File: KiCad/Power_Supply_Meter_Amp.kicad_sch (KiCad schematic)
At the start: 630 parts, among them J1 R_Phono_In, J10 VCC_IN, J11 VCC_OUT, J12 EMK_In, J13 EMK_Out, J14 EMK_Out, J15 Mic_Effekt_Out, J16 Mic_Effekt_Out, J17 Mic_Effekt_Out, J18 Mic_Effekt_Out, J19 Phono/Line_Out, J2 L_Phono_In, J20 Mic_Effekt_Out, J21 Conn_01x05_bridged, J22 EMK_In, J24 Mic_Effekt_In, J25 Mic_Effekt_In, J26 Phono/Line_In, J27 Mic_Effekt_In, J28 Pegel_Out, J29 Pegel_Out, J3 R_Line_In, J30 Pegel_In, J31 Pegel_In, J32 Pegel_In, J33 Pegel_In, J34 LED_Out, J35 LED_In, J36 VU_Meter_Out, J37 AUX_Send_3, J38 AUX_Send_1, J39 AUX_Send_2, J4 L_Line_In, J40 Bass_Out, J41 Kick_Out, J42 Mid_Out, J43 High_Out, J44 Line_Out_L, J45 Line_Out_R, J5 Mic_In, J6 Effekt_In, J7 AUX_RET_1, J8 AUX_RET_2, J9 AUX_RET_3, SW1 SW_DPST, SW10 SW_SPDT, SW11 SW_SPDT, SW12 SW_SPDT, SW2 SW_SPDT, SW3 SW_SPDT, SW4 SW_SPDT, SW5 SW_SPDT, SW6 SW_SPDT, SW7 SW_SPDT, SW8 SW_SPDT, SW9 SW_Rotary_1x4, U1 TL074, U10 TL074, U11 TL074, U12 TL074, U13 TL074, U14 TL074, U15 TL074, U16 TL074, U17 TL074, U18 TL074, U19 TL074, U2 TL074, U20 TL074, U21 TL074, U22 TL074, U23 TL074, U24 TL074, U25 INA128U, U3 TL074, U4 TL074, U5 TL074, U6 REC10K-2409, U7 REC10K-2415, U8 TL074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

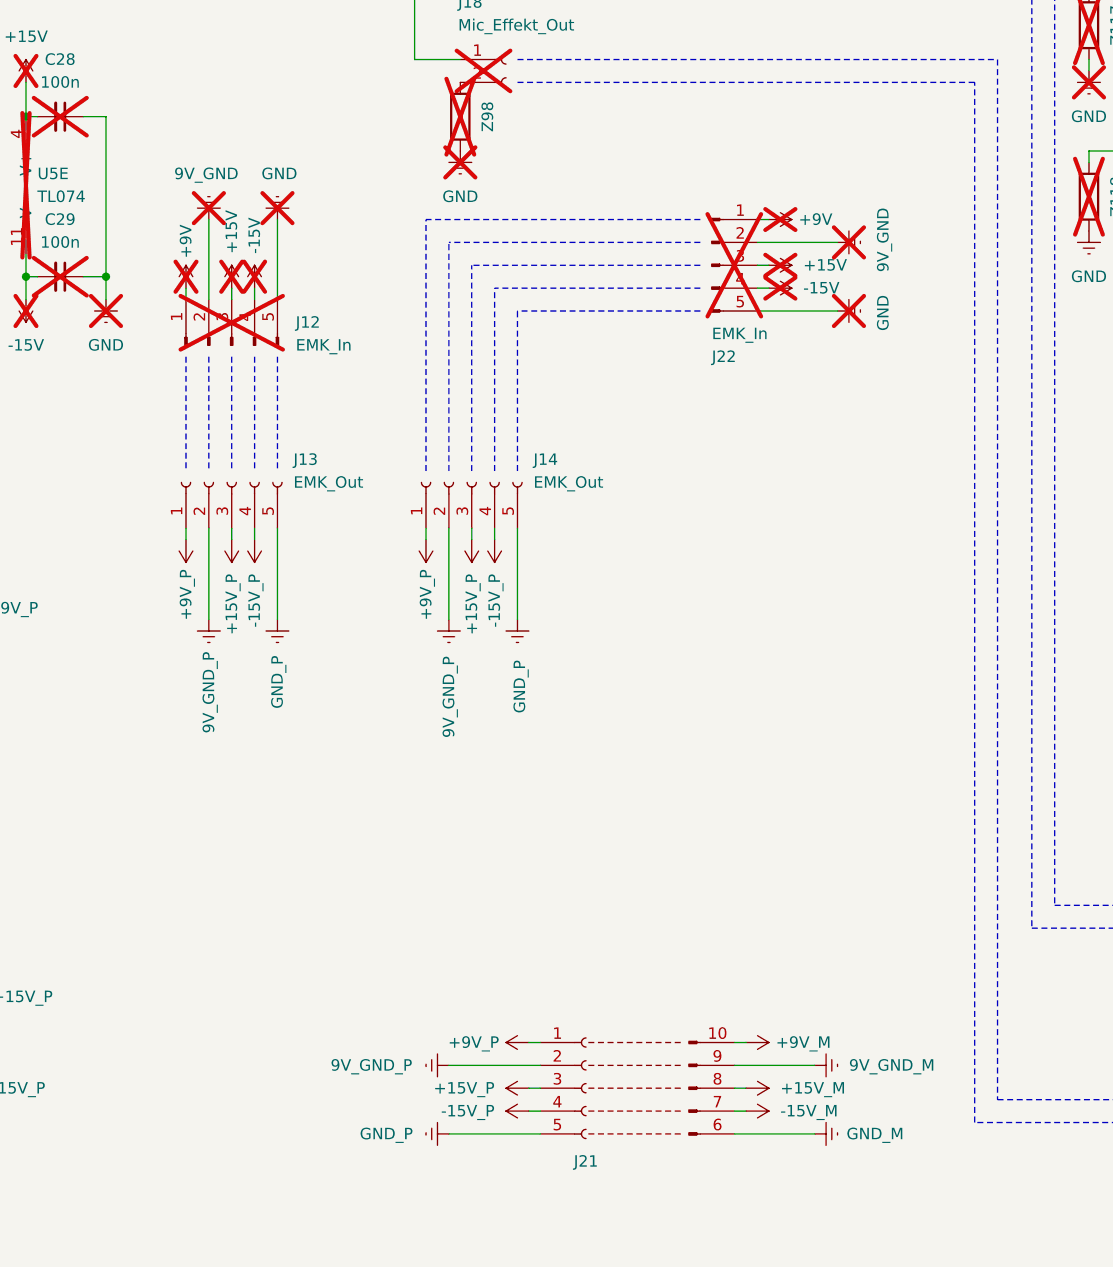
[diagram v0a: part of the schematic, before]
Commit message: PCB Update
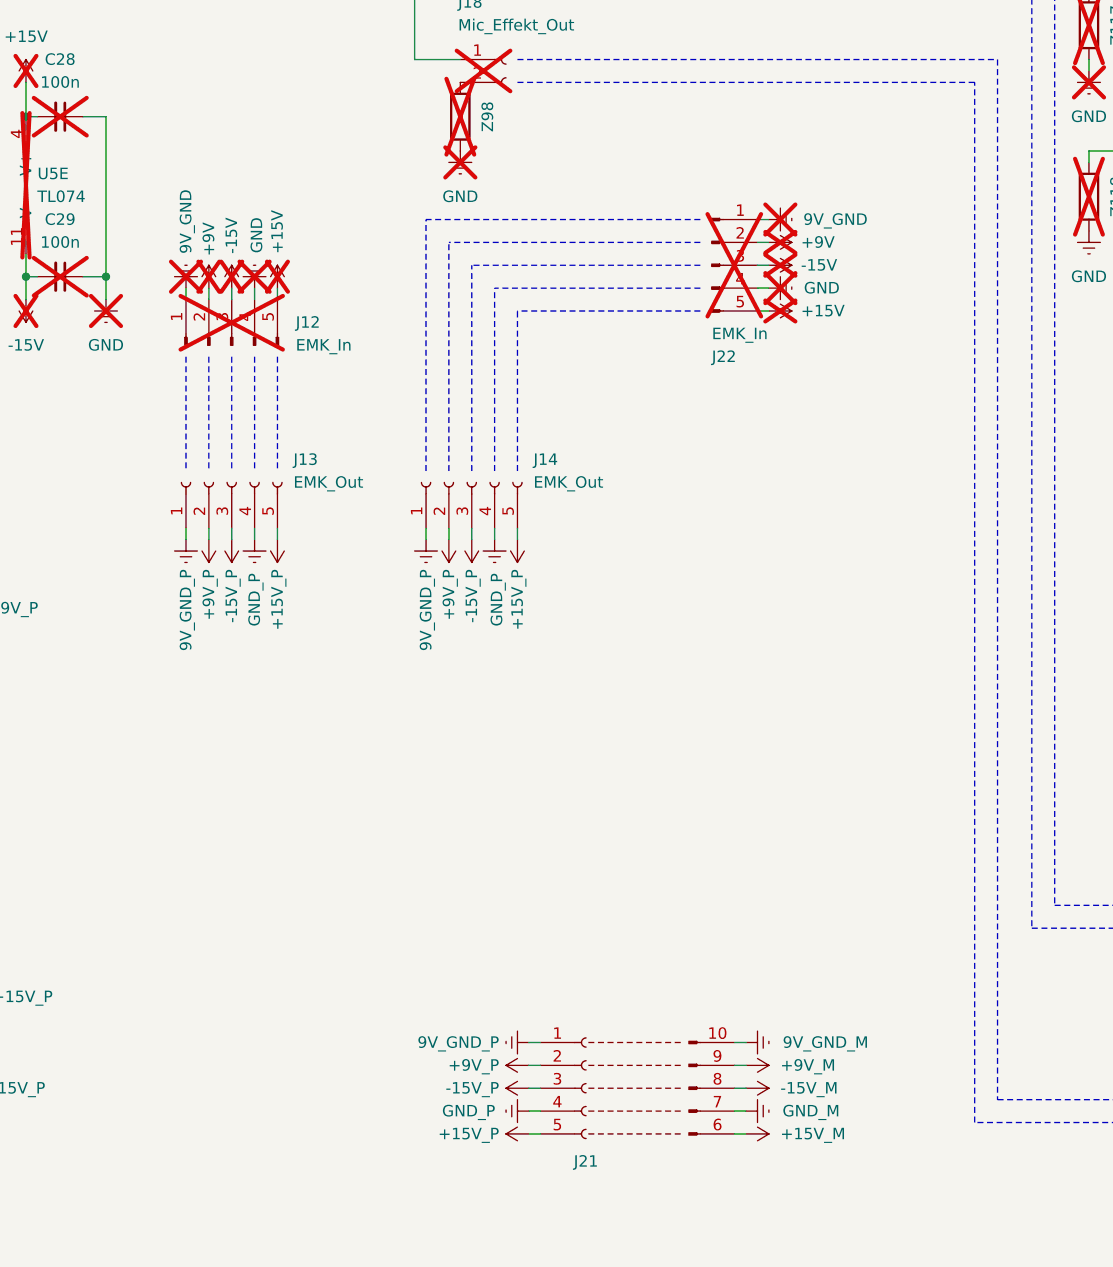
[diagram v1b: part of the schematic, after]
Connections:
- net +15V: now also J12.5 (Pin_5), J22.5 (Pin_5); no longer J12.3 (Pin_3), J22.3 (Pin_3)
- net +15V_M: now also J21.6 (Pin_5); no longer J21.8 (Pin_3)
- net +15V_P: now also J13.5 (Pin_5), J14.5 (Pin_5), J21.5 (Pin_5); no longer J13.3 (Pin_3), J14.3 (Pin_3), J21.3 (Pin_3)
- net +9V: now also J12.2 (Pin_2), J22.2 (Pin_2); no longer J12.1 (Pin_1), J22.1 (Pin_1)
- net +9V_M: now also J21.9 (Pin_2); no longer J21.10 (Pin_1)
- net +9V_P: now also J13.2 (Pin_2), J14.2 (Pin_2), J21.2 (Pin_2); no longer J13.1 (Pin_1), J14.1 (Pin_1), J21.1 (Pin_1)
- net -15V: now also J12.3 (Pin_3), J22.3 (Pin_3); no longer J12.4 (Pin_4), J22.4 (Pin_4)
- net -15V_M: now also J21.8 (Pin_3); no longer J21.7 (Pin_4)
- net -15V_P: now also J13.3 (Pin_3), J14.3 (Pin_3), J21.3 (Pin_3); no longer J13.4 (Pin_4), J14.4 (Pin_4), J21.4 (Pin_4)
- net 9V_GND: now also J12.1 (Pin_1), J22.1 (Pin_1); no longer J12.2 (Pin_2), J22.2 (Pin_2)
- net 9V_GND_M: now also J21.10 (Pin_1); no longer J21.9 (Pin_2)
- net 9V_GND_P: now also J13.1 (Pin_1), J14.1 (Pin_1), J21.1 (Pin_1); no longer J13.2 (Pin_2), J14.2 (Pin_2), J21.2 (Pin_2)
- net GND: now also J12.4 (Pin_4), J22.4 (Pin_4); no longer J12.5 (Pin_5), J22.5 (Pin_5)
- net GND_M: now also J21.7 (Pin_4); no longer J21.6 (Pin_5)
- net GND_P: now also J13.4 (Pin_4), J14.4 (Pin_4), J21.4 (Pin_4); no longer J13.5 (Pin_5), J14.5 (Pin_5), J21.5 (Pin_5)

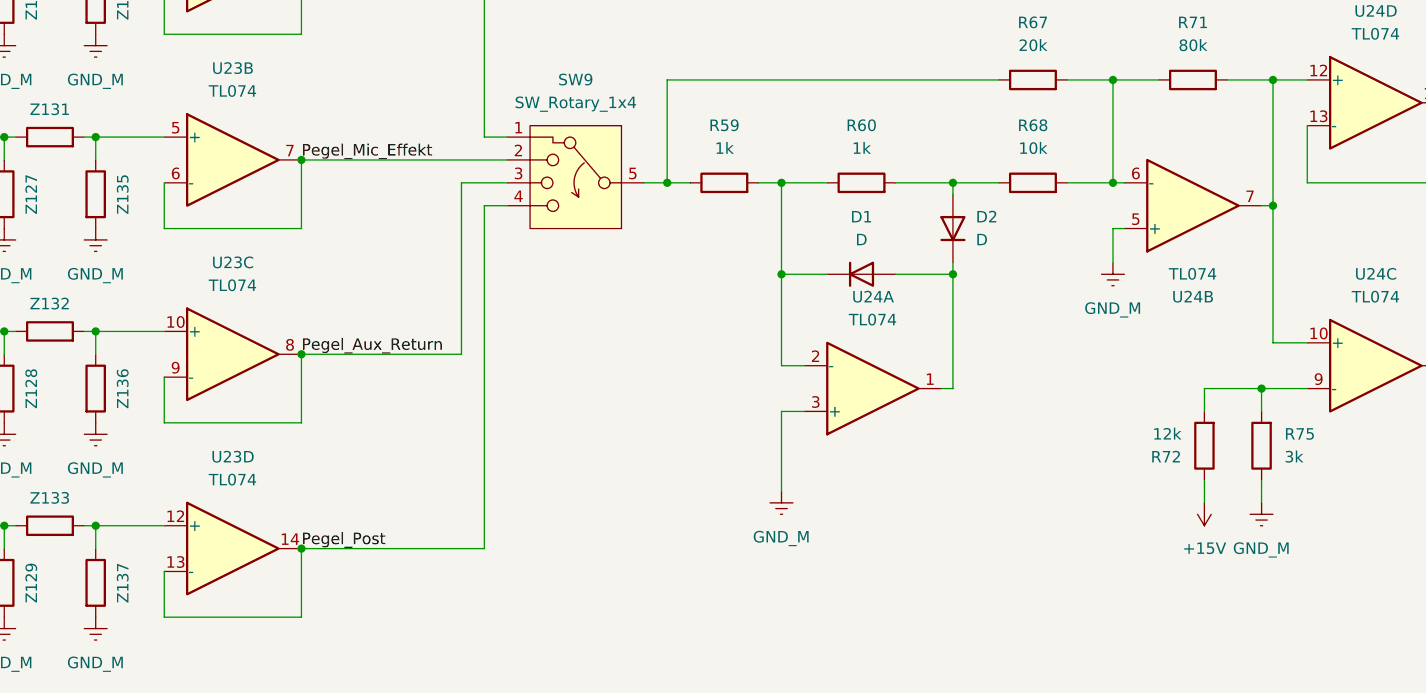
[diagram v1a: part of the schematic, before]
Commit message: PCB Update
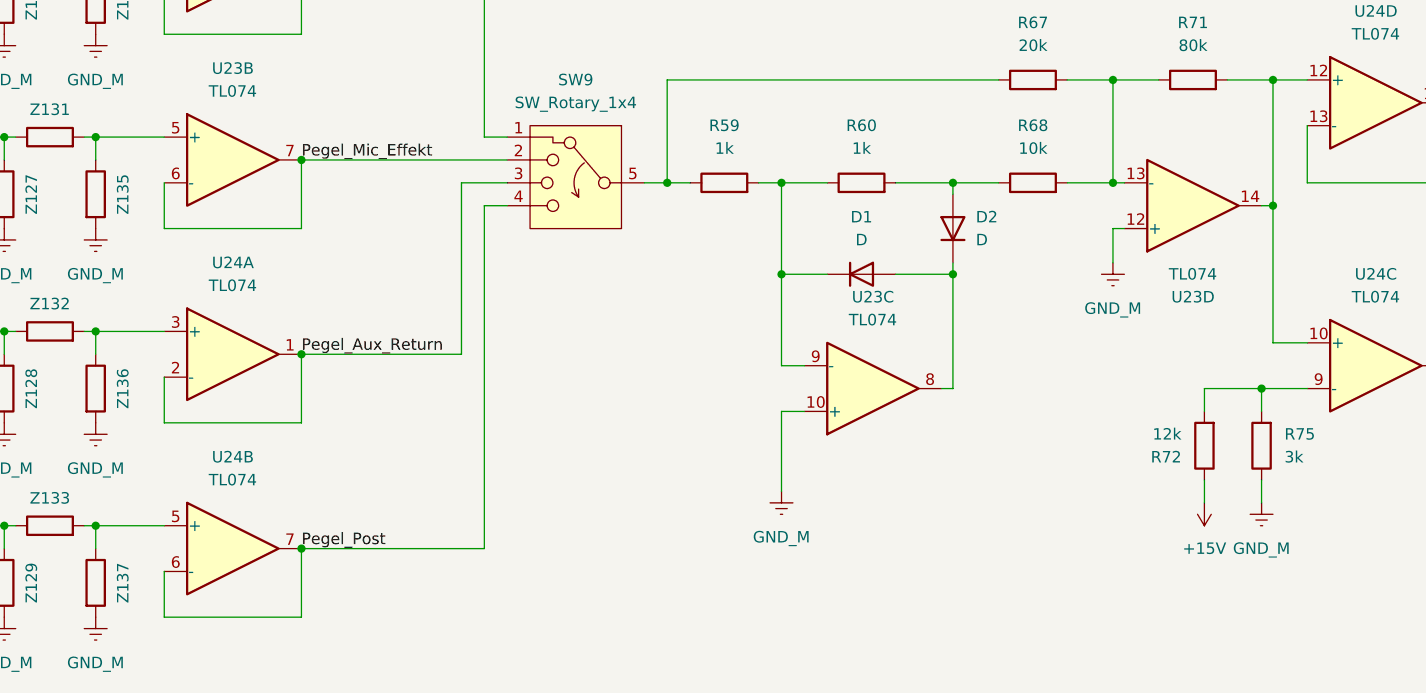
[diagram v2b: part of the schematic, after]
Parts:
- renumbered U24 to U23, U23 to U24
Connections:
- net GND_M: now also U23.10 (+), U23.12 (+); no longer U23.3 (+), U23.5 (+)
- net Pegel_Aux_Return: now also U24.1, U24.2 (-); no longer U24.8, U24.9 (-)
- net Pegel_Post: now also U24.6 (-), U24.7; no longer U24.13 (-), U24.14
- net at Z133.2, Z137.1: now also U24.5 (+); no longer U24.12 (+)
- net at D1.1 (K), R59.2, R60.1: now also U23.9 (-); no longer U23.2 (-)
- net at Z132.2, Z136.1: now also U24.3 (+); no longer U24.10 (+)
- net at D1.2 (A), D2.1 (K): now also U23.8; no longer U23.1
- net at R67.2, R68.2, R71.1: now also U23.13 (-); no longer U23.6 (-)
- net at R71.2, U24.10 (+), U24.12 (+): now also U23.14; no longer U23.7
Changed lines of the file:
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@@
 		(lib_id "Amplifier_Operational:TL074")
 		(at 438.15 541.02 0)
-		(unit 3)
+		(unit 1)
 		(exclude_from_sim no)
 		(in_bom yes)
 		(on_board yes)
 		(dnp no)
-		(property "Reference" "U23"
+		(property "Reference" "U24"
 			(at 438.15 530.86 0)
 			(effects
@@
 			(project ""
 				(path "/81a92cd6-862a-4567-ad33-f8a3bc120591"
-					(reference "U23")
-					(unit 3)
+					(reference "U24")
+					(unit 1)
 				)
 			)
@@
 		(at 509.27 544.83 0)
 		(mirror x)
-		(unit 1)
+		(unit 3)
 		(exclude_from_sim no)
 		(in_bom yes)
 		(on_board yes)
 		(dnp no)
-		(property "Reference" "U24"
+		(property "Reference" "U23"
 			(at 509.27 534.67 0)
 			(effects
@@
 			(project ""
 				(path "/81a92cd6-862a-4567-ad33-f8a3bc120591"
-					(reference "U24")
-					(unit 1)
+					(reference "U23")
+					(unit 3)
 				)
 			)
@@
 		(lib_id "Amplifier_Operational:TL074")
 		(at 438.15 562.61 0)
-		(unit 4)
+		(unit 2)
 		(exclude_from_sim no)
 		(in_bom yes)
@@
 		(dnp no)
 		(fields_autoplaced yes)
-		(property "Reference" "U23"
+		(property "Reference" "U24"
 			(at 438.15 552.45 0)
 			(effects
@@
 			(project "DiKo_PreAmp"
 				(path "/81a92cd6-862a-4567-ad33-f8a3bc120591"
-					(reference "U23")
-					(unit 4)
+					(reference "U24")
+					(unit 2)
 				)
 			)
@@
 		(at 544.83 524.51 0)
 		(mirror x)
-		(unit 2)
+		(unit 4)
 		(exclude_from_sim no)
 		(in_bom yes)
 		(on_board yes)
 		(dnp no)
-		(property "Reference" "U24"
+		(property "Reference" "U23"
 			(at 544.83 534.67 0)
 			(effects
@@
 			(project ""
 				(path "/81a92cd6-862a-4567-ad33-f8a3bc120591"
-					(reference "U24")
-					(unit 2)
+					(reference "U23")
+					(unit 4)
 				)
 			)
